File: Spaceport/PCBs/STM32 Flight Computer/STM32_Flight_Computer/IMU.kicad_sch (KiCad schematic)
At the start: 1 part, among them U1 BMI088

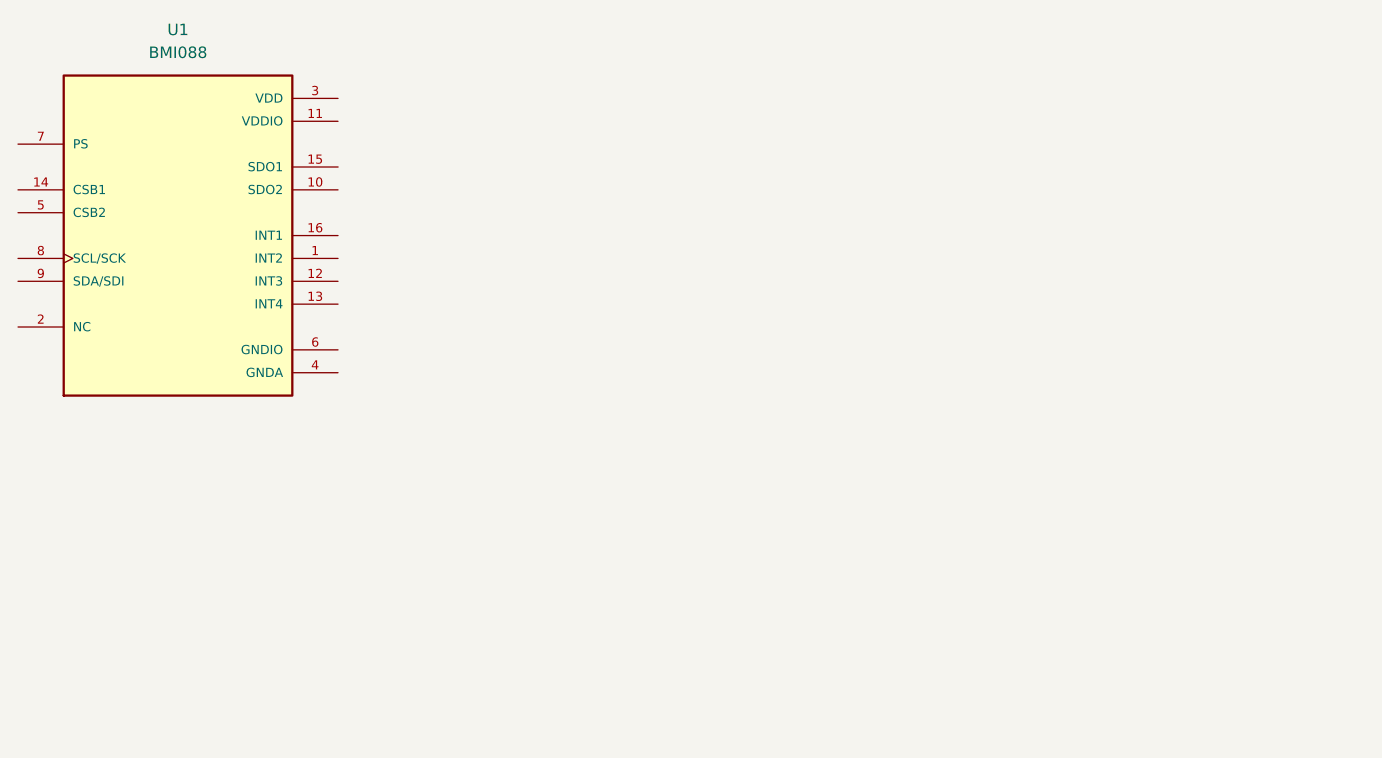
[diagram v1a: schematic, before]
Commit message: Subcircuit Updates
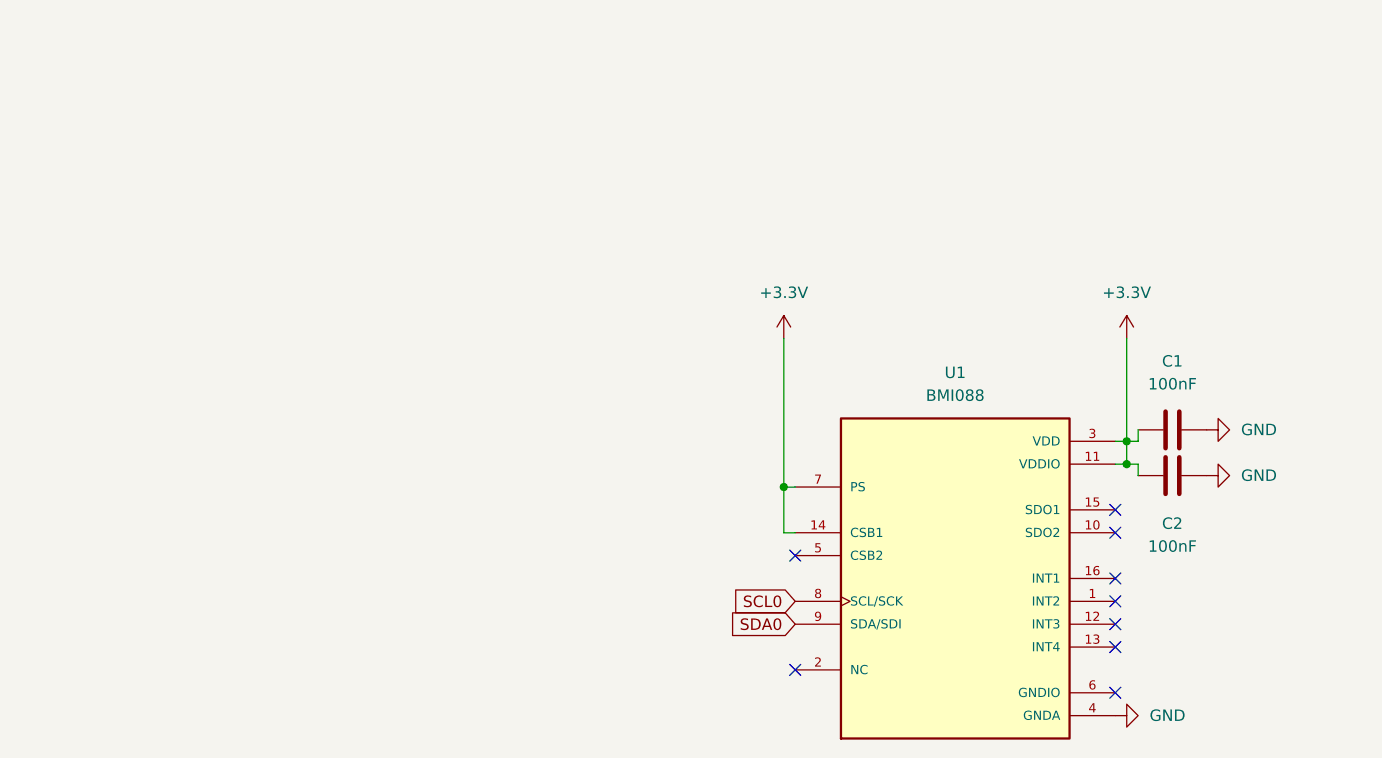
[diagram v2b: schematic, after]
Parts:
- added C1, C2: 100nF, symbol Device:C
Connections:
- net +3.3V: now reaches U1.11 (VDDIO)
- net +3.3V: now also U1.14 (CSB1), U1.3 (VDD), U1.7 (PS), C1.1, C2.2
- net GND: now reaches U1.4 (GNDA)
- net GND: now also C1.2, C2.1
- net SCL0: now reaches U1.8 (SCL/SCK)
- net SDA0: now reaches U1.9 (SDA/SDI)
- no-connect marks 0 -> 9
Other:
- moved on the sheet: U1

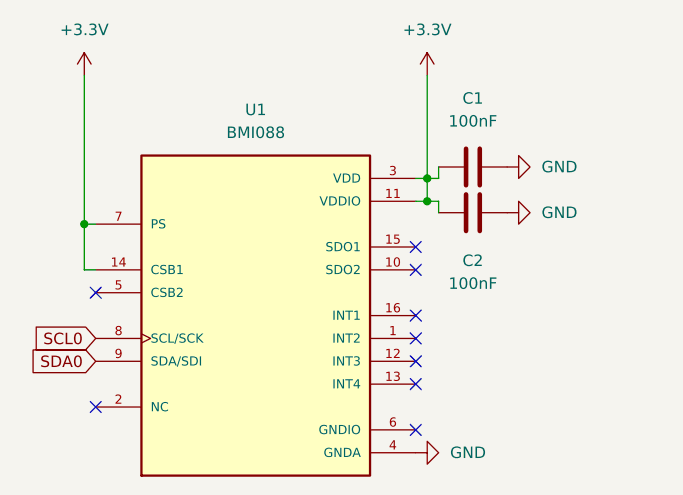
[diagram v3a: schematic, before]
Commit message: Push after Schematic Review 5/5
- Updated STM32 symbol
- Configured I2C busses
- Updated DC caps to 100nF
- TODO add power system things
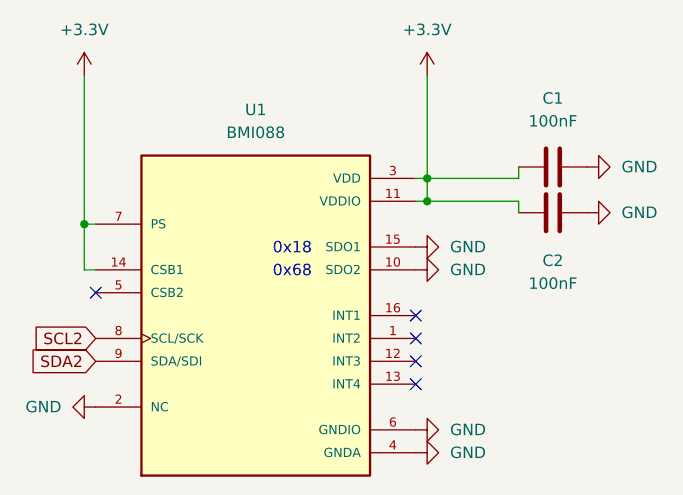
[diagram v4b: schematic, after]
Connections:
- net GND: now also U1.10 (SDO2), U1.15 (SDO1), U1.2 (NC), U1.6 (GNDIO)
- net SCL0 renamed SCL2
- net SDA0 renamed SDA2
- no-connect marks 9 -> 5
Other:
- note added: "0x18"
- note added: "0x68"
- moved on the sheet: C1, C2
